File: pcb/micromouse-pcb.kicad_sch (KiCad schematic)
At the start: 51 parts, among them J1 Conn_01x08, J1_MotorEncoder1 Conn_01x06, J2_MotorEncoder1 Conn_01x06, J3 Conn_01x08, J4 Conn_01x08, Q1 BS170, Q2 TEFT4300, Q3 BS170, Q4 TEFT4300, Q5 BS170, Q6 TEFT4300, Q7 BS170, Q8 TEFT4300, SW1 SW_SPDT, U1 Teensy_4.1, U2 L7805

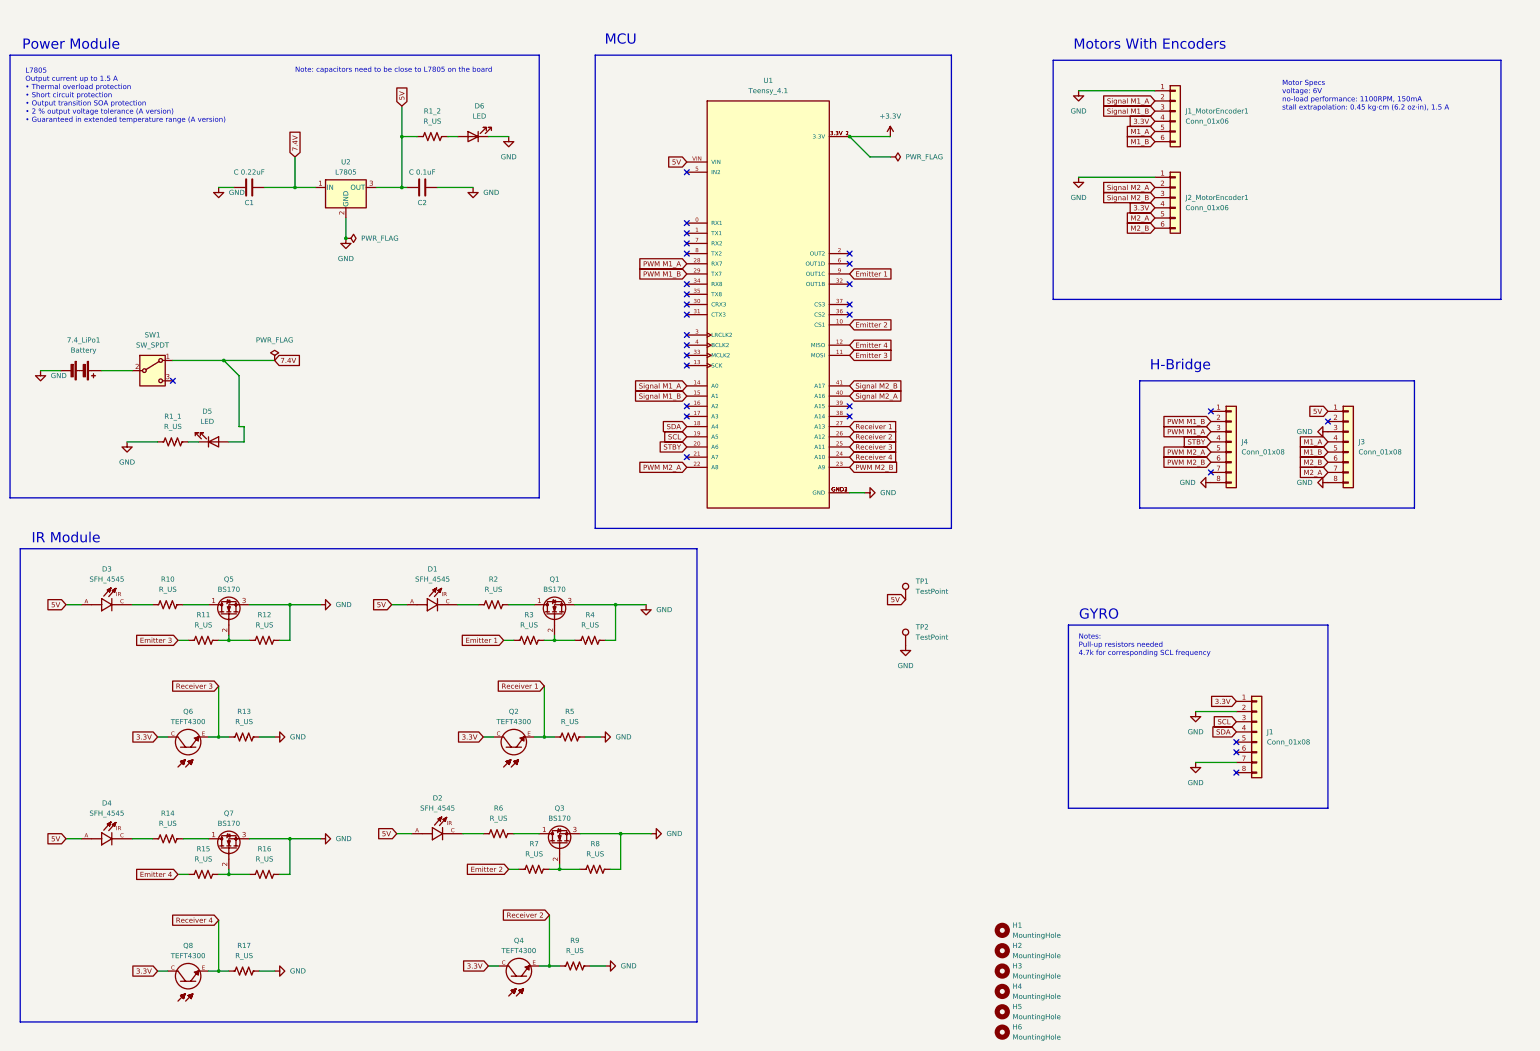
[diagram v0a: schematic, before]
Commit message: Done placement
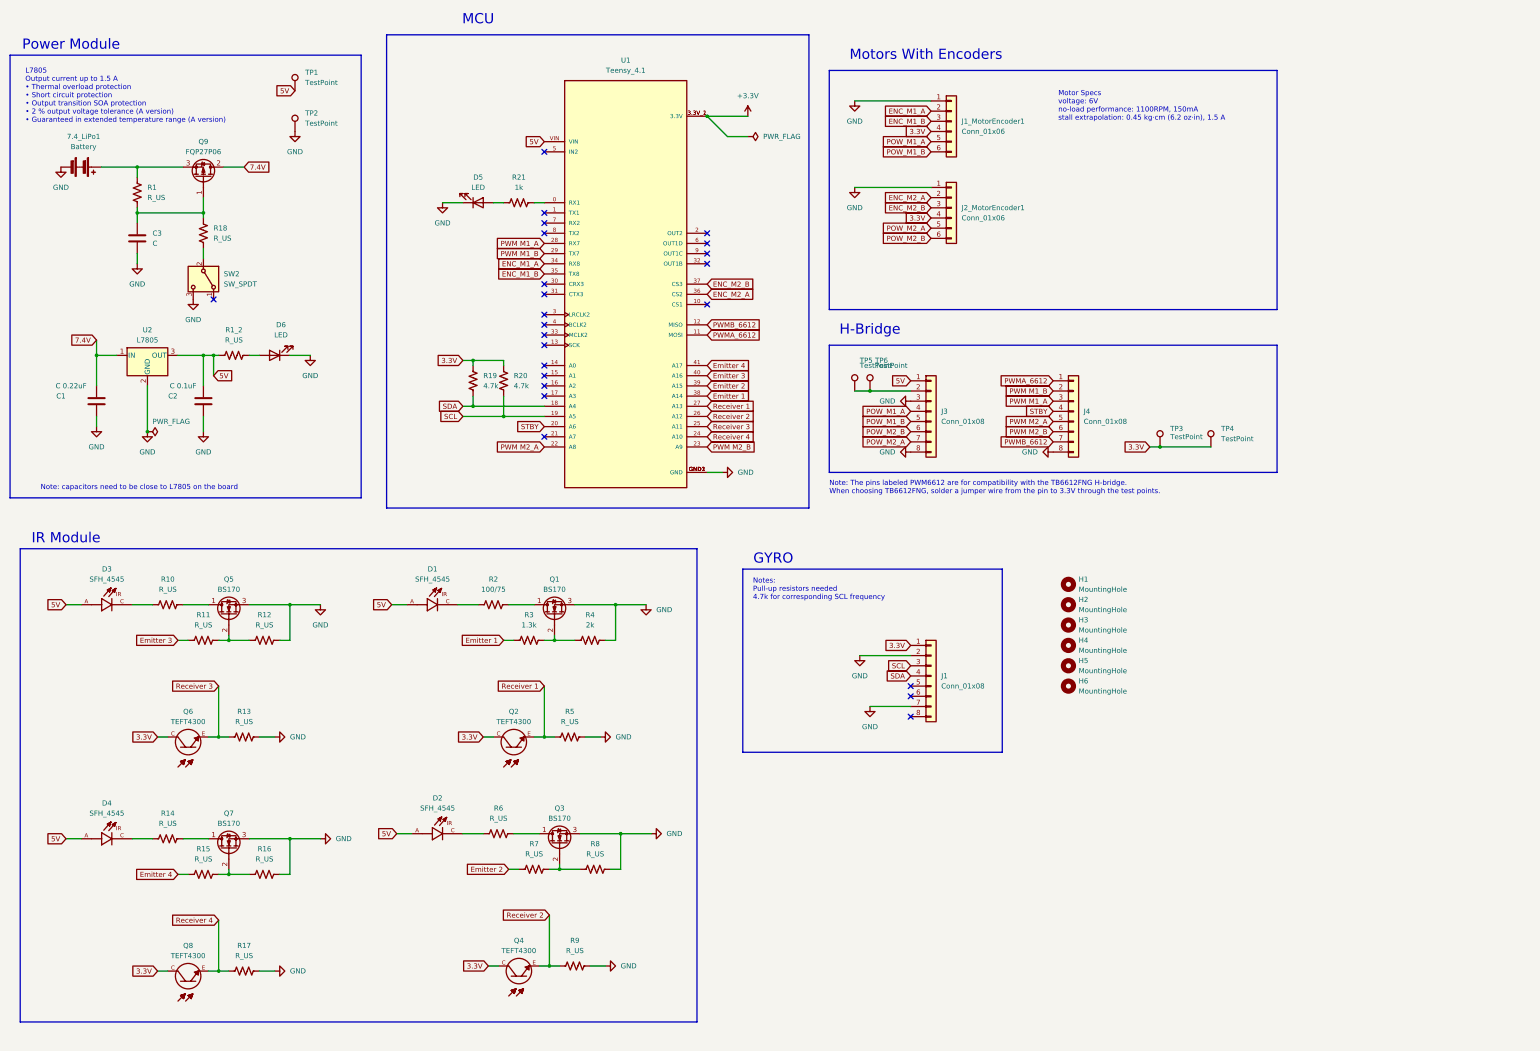
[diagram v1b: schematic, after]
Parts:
- removed R1_1: R_US, Resistor_SMD:R_1206_3216Metric_Pad1.30x1.75mm_HandSolder, symbol Device:R_US
- removed SW1: SW_SPDT, Connector_PinHeader_2.54mm:PinHeader_1x03_P2.54mm_Vertical, symbol Switch:SW_SPDT
- added C3: C, Capacitor_SMD:C_1206_3216Metric_Pad1.33x1.80mm_HandSolder, symbol Device:C
- added Q9: FQP27P06, Package_TO_SOT_THT:TO-220-3_Vertical, symbol Transistor_FET:FQP27P06
- added R1, R18: R_US, Resistor_SMD:R_1206_3216Metric_Pad1.30x1.75mm_HandSolder, symbol Device:R_US
- added R19, R20: 4.7k, Resistor_SMD:R_1206_3216Metric_Pad1.30x1.75mm_HandSolder, symbol Device:R_US
- added R21: 1k, Resistor_SMD:R_1206_3216Metric_Pad1.30x1.75mm_HandSolder, symbol Device:R_US
- added SW2: SW_SPDT, Button_Switch_THT:SW_Slide_SPDT_Angled_CK_OS102011MA1Q, symbol Switch:SW_SPDT
- added TP3, TP4, TP5, TP6: TestPoint, micromouse:TestPoint_THTPad_D2.0mm_Drill1.0mm, symbol Connector:TestPoint
- 7.4_LiPo1: footprint Connector_PinHeader_2.54mm:PinHeader_1x02_P2.54mm_Vertical -> Connector_JST:JST_PH_B2B-PH-K_1x02_P2.00mm_Vertical
- D1, D2, D3, D4: footprint micromouse:LED_D5.0mm_IR -> micromouse:DIO_SFH_4545_copy
- D5, D6: footprint LED_THT:LED_D5.0mm -> LED_SMD:LED_1206_3216Metric_Pad1.42x1.75mm_HandSolder
- R2: value R_US -> 100/75
- R3: value R_US -> 1.3k
- R4: value R_US -> 2k
- TP1, TP2: footprint TestPoint:TestPoint_THTPad_D1.5mm_Drill0.7mm -> micromouse:TestPoint_THTPad_D2.0mm_Drill1.0mm
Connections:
- net 3.3V: now also R19.1, R20.1, TP3.1, TP4.1
- net 5V: now also C2.2; no longer C2.1
- net 7.4V: now also Q9.2 (D); no longer D5.2 (A)
- net Emitter 1: now also U1.38 (A14); no longer U1.9 (OUT1C)
- net Emitter 2: now also U1.39 (A15); no longer U1.10 (CS1)
- net Emitter 3: now also U1.40 (A16); no longer U1.11 (MOSI)
- net Emitter 4: now also U1.41 (A17); no longer U1.12 (MISO)
- net GND: now also C2.1, D5.1 (K), C3.2, SW2.3 (C); no longer C2.2
- net SCL: now also R20.2
- net SDA: now also R19.2
- net at U1.0 (RX1): now also R21.2
- net ENC_M1_A: now reaches U1.34 (RX8)
- net ENC_M1_A: now also J1_MotorEncoder1.2 (Pin_2)
- net ENC_M1_B: now reaches U1.35 (TX8)
- net ENC_M1_B: now also J1_MotorEncoder1.3 (Pin_3)
- net ENC_M2_A: now reaches U1.36 (CS2)
- net ENC_M2_A: now also J2_MotorEncoder1.2 (Pin_2)
- net ENC_M2_B: now reaches U1.37 (CS3)
- net ENC_M2_B: now also J2_MotorEncoder1.3 (Pin_3)
- net at 7.4_LiPo1.1 (+): now also Q9.3 (S), R1.1
- net at J3.2 (Pin_2): now also TP5.1, TP6.1
- net PWMA_6612: now reaches J4.1 (Pin_1)
- net PWMA_6612: now also U1.11 (MOSI)
- net PWMB_6612: now reaches J4.7 (Pin_7)
- net PWMB_6612: now also U1.12 (MISO)
- net M1_A renamed POW_M1_A
- net M1_B renamed POW_M1_B
- net M2_A renamed POW_M2_A
- net M2_B renamed POW_M2_B
- net Signal M1_A: no longer names the net of U1.14 (A0)
- net Signal M1_A: no longer J1_MotorEncoder1.2 (Pin_2)
- net Signal M1_B: no longer names the net of U1.15 (A1)
- net Signal M1_B: no longer J1_MotorEncoder1.3 (Pin_3)
- removed net Signal M2_A: J2_MotorEncoder1.2 (Pin_2), U1.40 (A16)
- removed net Signal M2_B: J2_MotorEncoder1.3 (Pin_3), U1.41 (A17)
- new net: C3.1, Q9.1 (G), R1.2, R18.1
- new net: R18.2, SW2.2 (B)
- new net: D5.2 (A), R21.1
- no-connect marks 30 -> 24
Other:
- note added: "Note: The pins labeled PWM6612 are for compatibility with the TB6612FNG H-bridge. When choosing TB6612FNG, solder a jumper wire from the pin to 3.3V through the test points."
- moved on the sheet: C1, C2, D6, H1, H2, H3, H4, H5, H6, J1, J1_MotorEncoder1, J2_MotorEncoder1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
